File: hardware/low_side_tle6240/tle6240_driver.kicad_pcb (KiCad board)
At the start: 2 copper layers, 42.7 x 56.5 mm, 12 parts, among them K1 JUMPER3, K2 CONN_3, P1 CONN_10X2, P2 CONN_16, P3 CONN_2X2

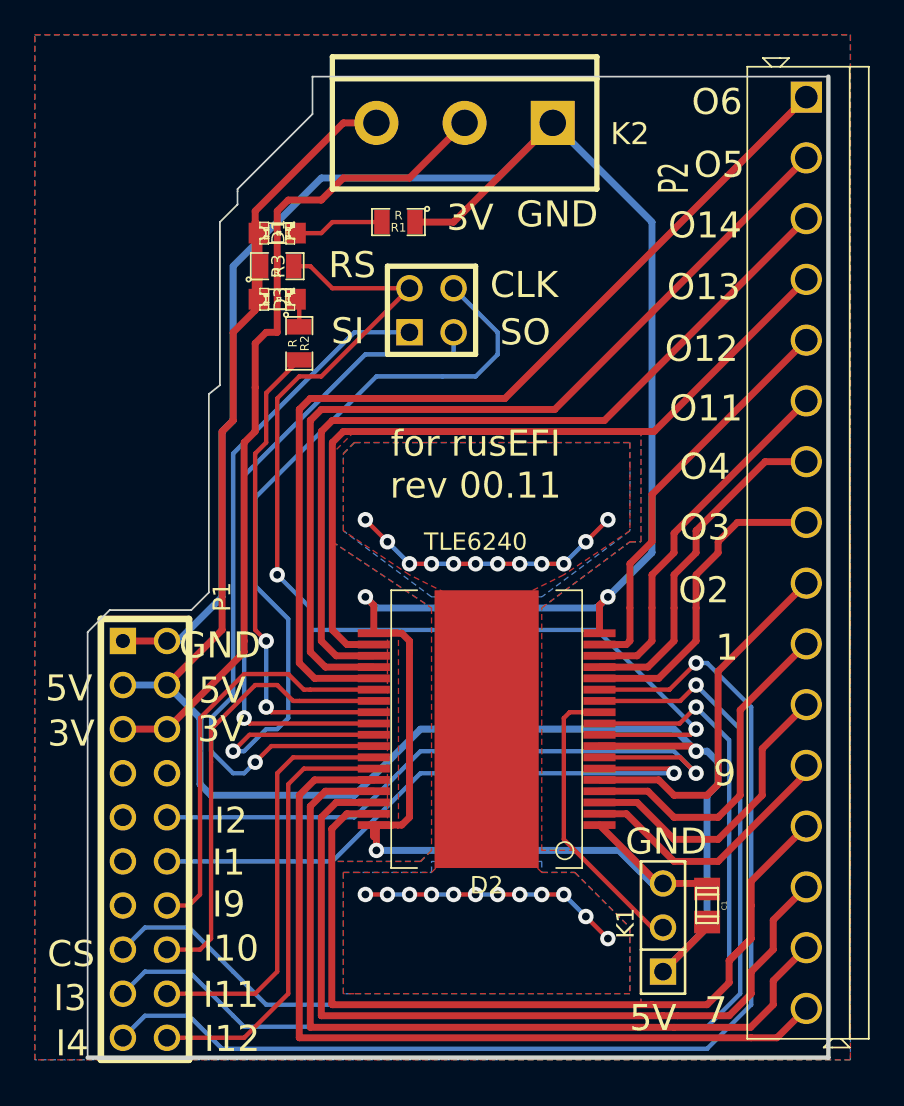
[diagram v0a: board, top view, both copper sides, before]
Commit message: update pcb files
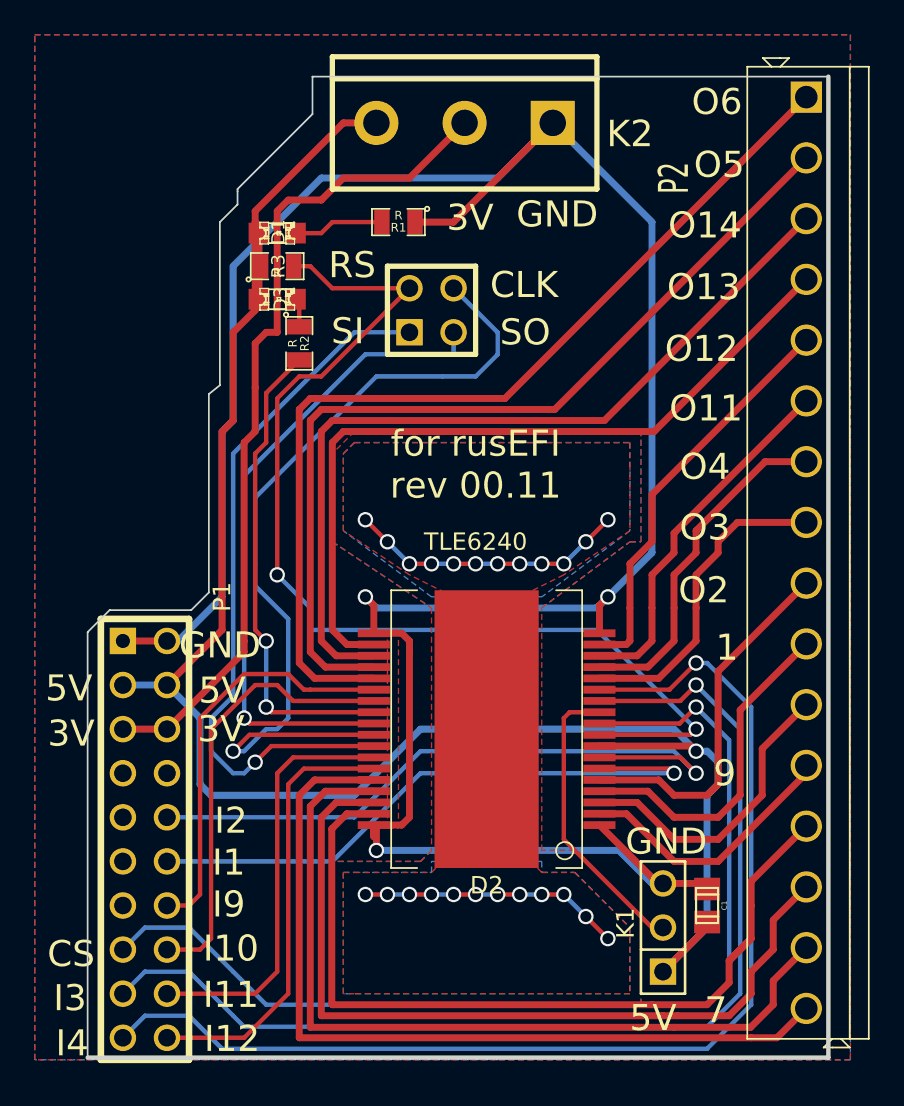
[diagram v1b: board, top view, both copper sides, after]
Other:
- net class Default removed
- net class Power removed
- net class Signal removed
